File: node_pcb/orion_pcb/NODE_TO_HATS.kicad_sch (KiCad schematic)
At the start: 0 parts

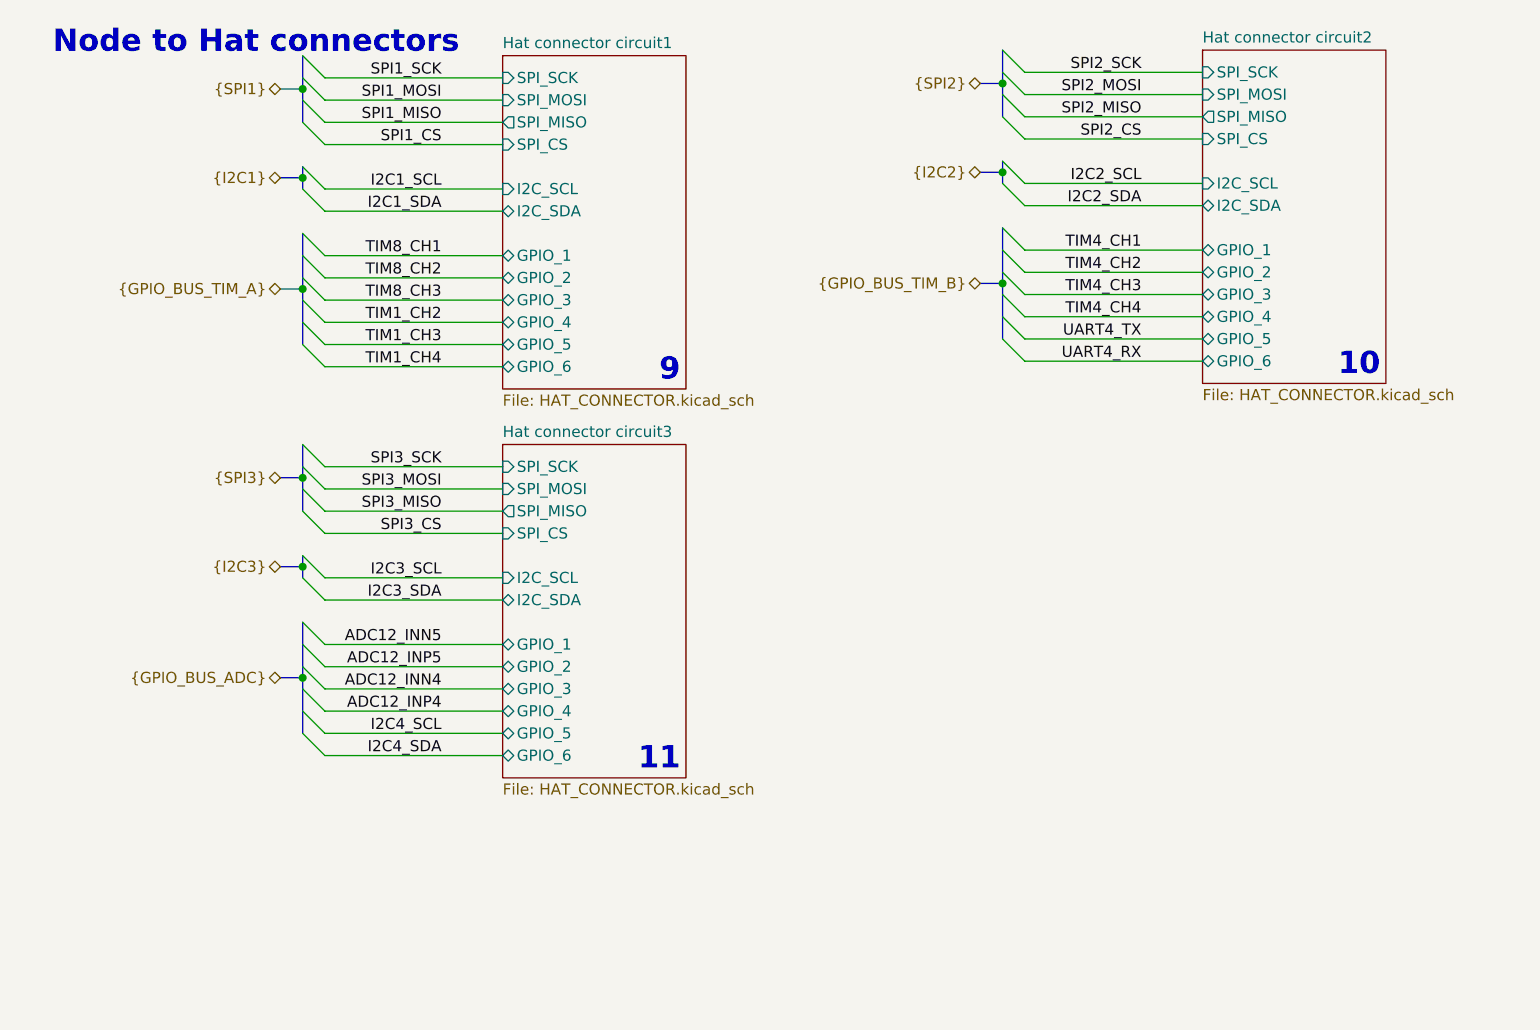
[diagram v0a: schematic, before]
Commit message: Added orion rev2 (no teardrops/rounded traces)
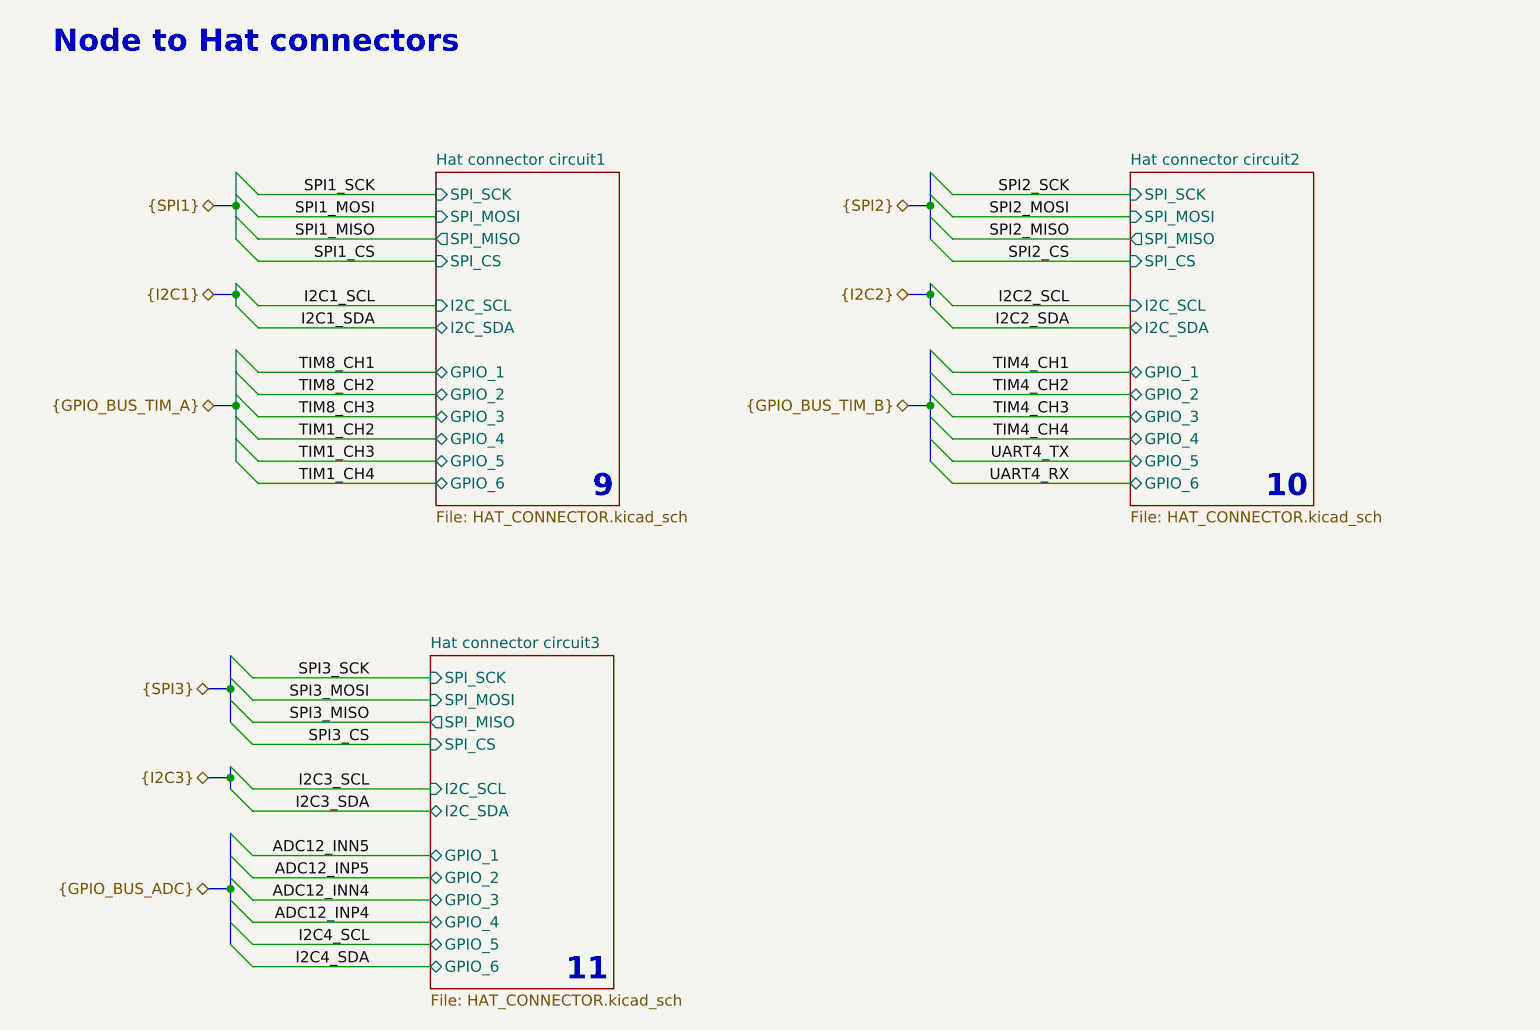
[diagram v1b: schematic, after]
